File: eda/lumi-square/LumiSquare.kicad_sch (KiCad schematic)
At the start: 102 parts, among them J1 USB_C_Receptacle_USB2.0_14P, J2 Conn_01x12, J3 Conn_01x12, J5 Conn_01x08, J6 Conn_01x08, J7 FTSH-105-01-X-DV-P-K-X, Q1 IRLML6244, Q10 IRLML2246, Q15 TSM680P06CH, Q16 TSM680P06CH, Q17 TSM680P06CH, Q18 TSM680P06CH, Q2 IRLML2246, Q3 IRLML2246, Q4 MMBT3904, Q5 MMBT3904, Q6 MMBT3904, Q7 MMBT3904, Q8 MMBT3904, Q9 MMBT3904, SW1 SW_SPST, SW2 SW_Push, SW3 SW_Push, SW4 SW_Push, SW5 SW_Push, U1 MCP73831-2-OT, U2 TPS3840, U3 TLV61070A, U4 TLV61070A, U5 ATSAMD21J18A-A, U6 STP16CPC05MTR, U7 CM1224-02SR, U8 MIC5225-3.3YM5

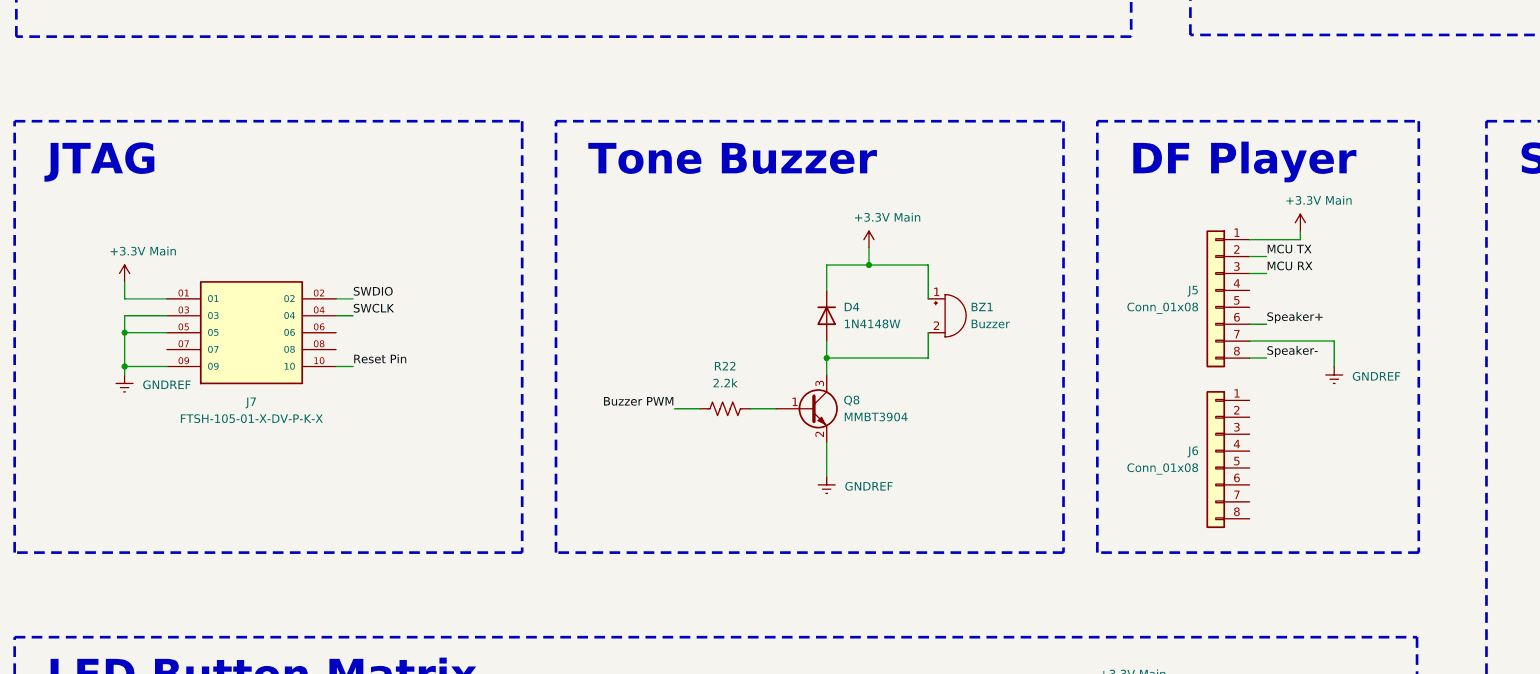
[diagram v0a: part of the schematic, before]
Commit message: Adding updateds to pcb and schematic design
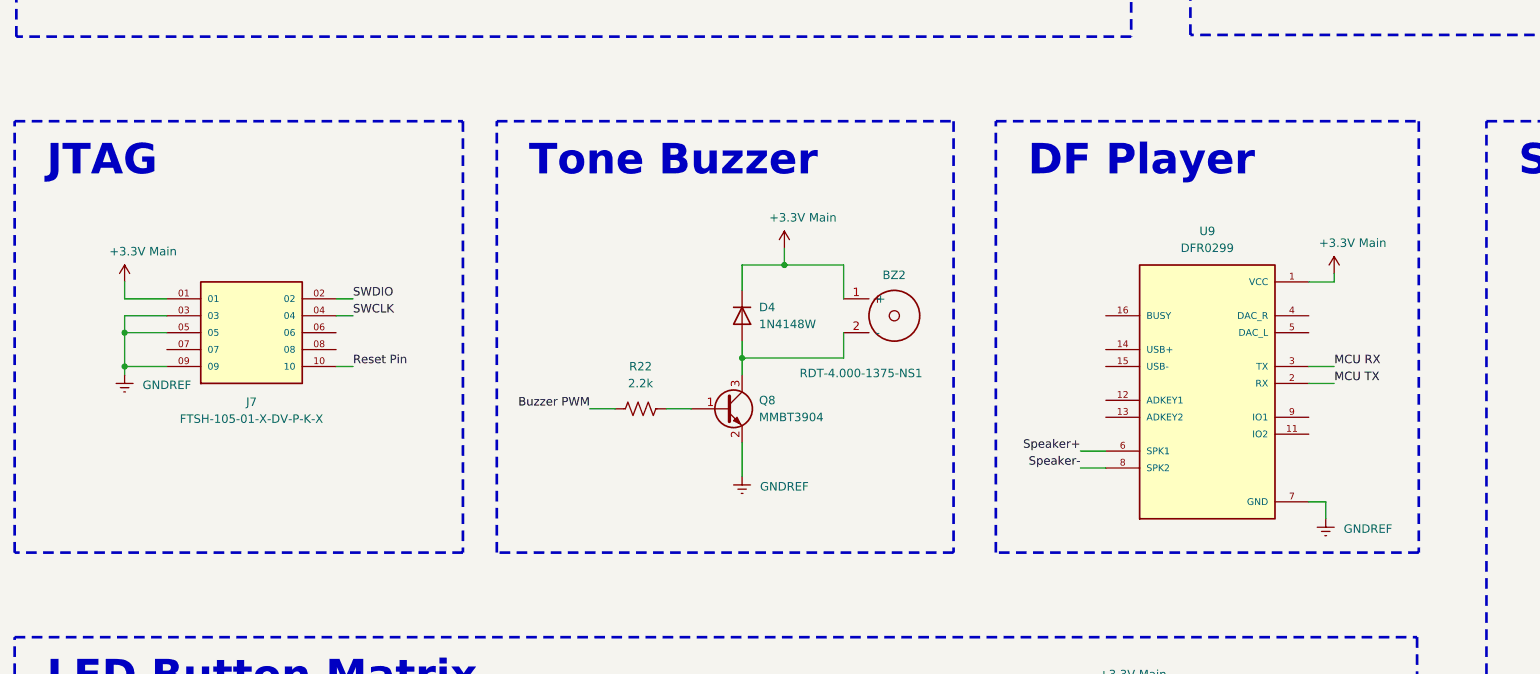
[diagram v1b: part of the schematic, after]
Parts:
- removed BZ1: Buzzer, symbol Device:Buzzer
- removed J5, J6: Conn_01x08, Connector_PinSocket_2.54mm:PinSocket_1x08_P2.54mm_Vertical, symbol Connector_Generic:Conn_01x08
- added BZ2: RDT-4.000-1375-NS1, RDT.pretty:RDT-4.000-1375-NS1, symbol RDT-4.000-1375-NS1:RDT-4.000-1375-NS1
- added U9: DFR0299, DFR0299:MODULE_DFR0299, symbol DFR0299:DFR0299
- C13, C14, C15, C16, C17, C18, C19, C20, C21: footprint Capacitor_SMD:C_0201_0603Metric_Pad0.64x0.40mm_HandSolder -> Capacitor_SMD:C_0603_1608Metric_Pad1.08x0.95mm_HandSolder
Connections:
- net +3.3V Main: now also BZ2.1 (+), U9.1 (VCC)
- net MCU RX: now also U9.3 (TX)
- net MCU TX: now also U9.2 (RX)
- net Speaker+: now also U9.6 (SPK1)
- net Speaker-: now also U9.8 (SPK2)
- net at D4.2 (A), Q8.3 (C): now also BZ2.2 (-)
- net GNDREF renamed GND
- net GND: now also U9.10 (GND), U9.7 (GND)
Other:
- moved on the sheet: D4, Q8, R22
